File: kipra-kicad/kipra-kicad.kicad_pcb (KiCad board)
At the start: 2 copper layers, 128.2 x 134.8 mm, 51 parts

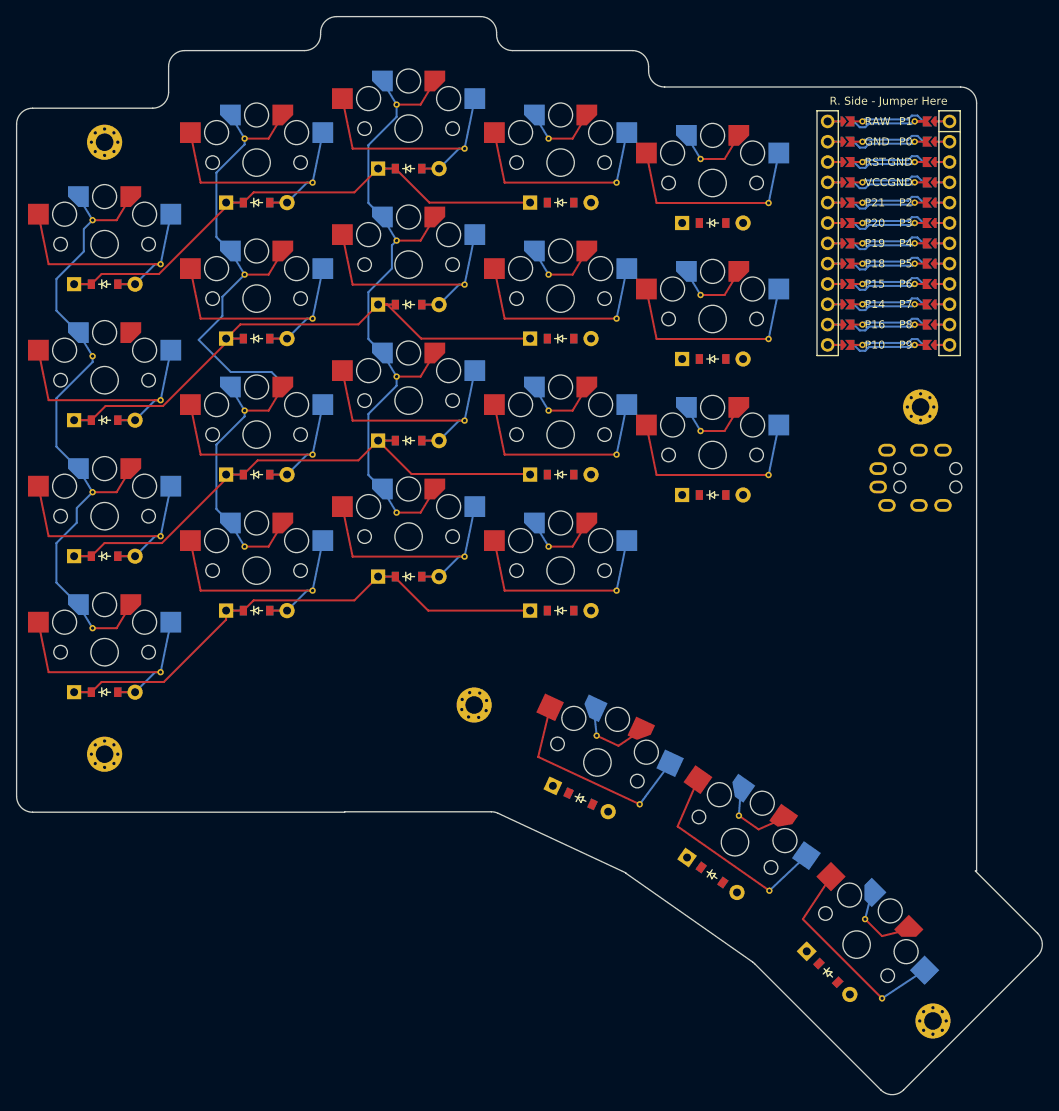
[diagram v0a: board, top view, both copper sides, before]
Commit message: I think maybe I just need ground now
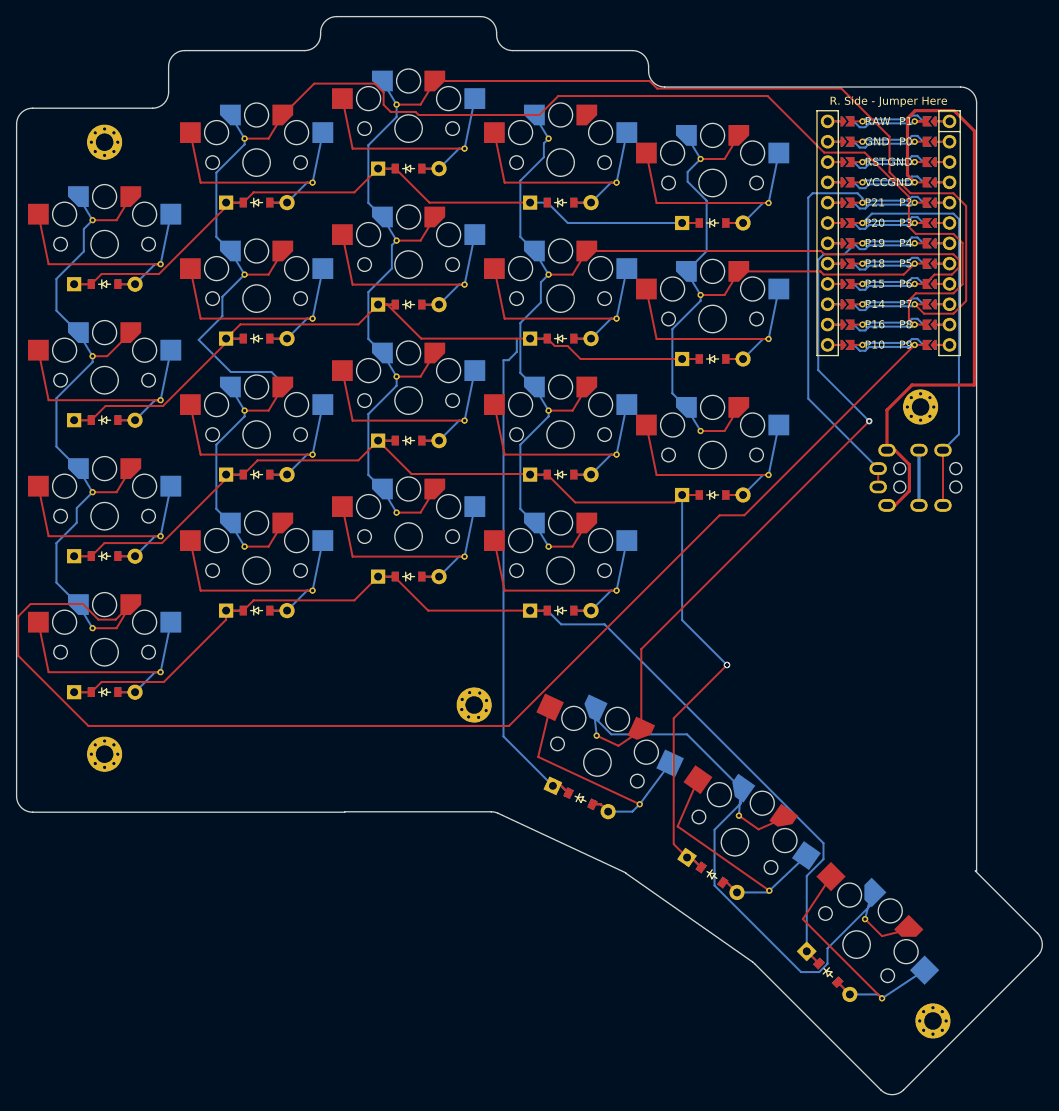
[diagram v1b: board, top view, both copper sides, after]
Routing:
- net P10: track 94.5 -> 257.1 mm
- net P19: track 39.8 -> 185.2 mm, vias 0 -> 1
- net P16: track 105.0 -> 221.0 mm
- net P15: track 49.7 -> 144.9 mm
- net P14: track 98.4 -> 193.4 mm
- net P06: track 75.9 -> 166.6 mm
- net P07: track 73.7 -> 156.7 mm, vias 0 -> 2
- net VCC: track 10.2 -> 87.7 mm
- net P08: track 72.0 -> 141.6 mm
- net P18: track 39.8 -> 95.6 mm
- net P3: track 10.2 -> 59.6 mm
- net P2: track 10.2 -> 57.8 mm
- net P05: track 71.5 -> 95.9 mm
- net thumb_near: track 26.8 -> 35.8 mm
- net thumb_middle: track 26.8 -> 35.5 mm
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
